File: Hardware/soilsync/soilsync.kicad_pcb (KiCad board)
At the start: 2 copper layers, 40 parts, among them J1 Barrel_Jack_Switch, J10 Screw_Terminal_01x03, J11 Screw_Terminal_01x03, J12 Screw_Terminal_01x03, J14 BMS_Terminal, J2 Screw_Terminal_01x03, J3 Screw_Terminal_01x03, J4 Screw_Terminal_01x03, J5 Screw_Terminal_01x03, J6 Screw_Terminal_01x03, J7 Screw_Terminal_01x03, J8 Screw_Terminal_01x03, J9 Screw_Terminal_01x03, U1 STM32F103C8Tx, U2 LM2596, U3 NRF24L01_Breakout, U4 AMS1117-3.3, U5 TP5100

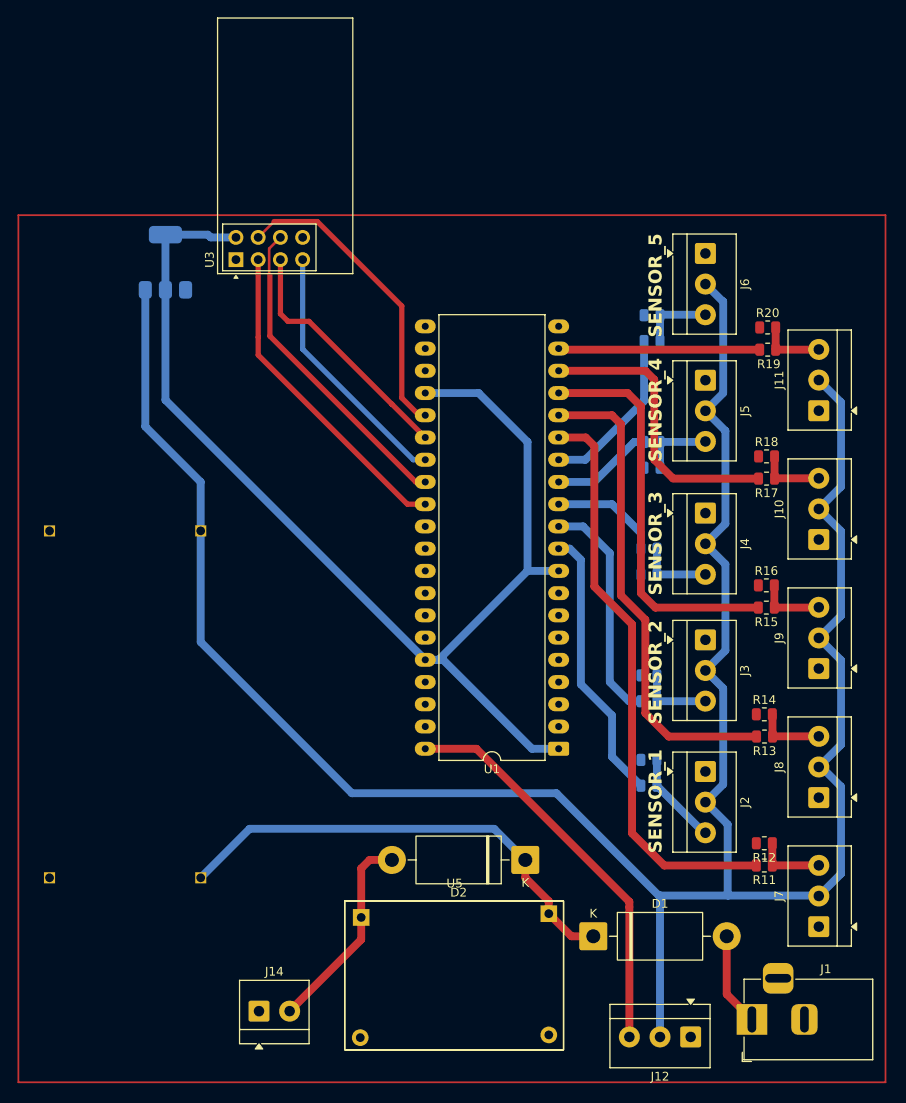
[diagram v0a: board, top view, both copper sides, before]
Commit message: PCB Finished
Generated fabrication data
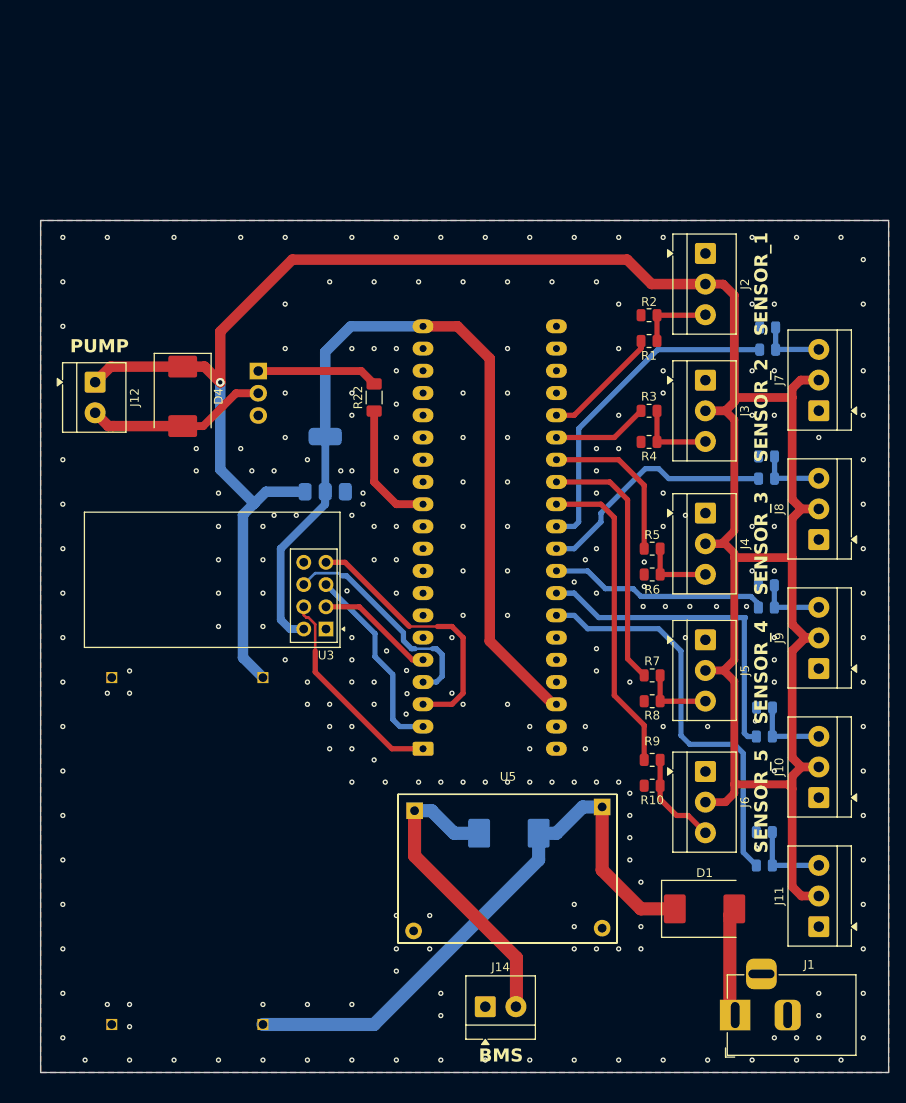
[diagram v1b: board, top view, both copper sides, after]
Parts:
- added D4: MBRS340, Diode_SMD:D_SMC, F.Cu at (183.9, 47.4)
- added Q1: IRLZ44N, Package_TO_SOT_THT:TO-220-3_Vertical, B.Cu at (192.5, 44.5)
- added R22: 100, Resistor_SMD:R_1206_3216Metric_Pad1.30x1.75mm_HandSolder, F.Cu at (205.7, 47.5)
- D1: value MBR340 -> MBRS340; footprint Diode_THT:D_DO-201AD_P15.24mm_Horizontal -> Diode_SMD:D_SMC
- D2: value MBR340 -> MBRS340; footprint Diode_THT:D_DO-201AD_P15.24mm_Horizontal -> Diode_SMD:D_SMC; moved to B.Cu
- J12: value Screw_Terminal_01x03 -> PUMP_Terminal; footprint TerminalBlock_4Ucon:TerminalBlock_4Ucon_1x03_P3.50mm_Horizontal -> TerminalBlock_4Ucon:TerminalBlock_4Ucon_1x02_P3.50mm_Horizontal
- R1, R10, R2, R3, R4, R5, R6, R7, R8, R9: moved to F.Cu
- R11, R12, R13, R14, R15, R16, R17, R18, R19, R20: moved to B.Cu
- U1: value STM32F103C8Tx -> YAAJ_BluePill; moved to B.Cu
- moved J12 101.1 mm to (173.9, 45.7), turned to -90 degrees
- moved J2 59.2 mm to (243.6, 31.0)
- moved J6 59.2 mm to (243.6, 90.2)
- moved J11 58.9 mm to (256.5, 108.0)
- moved J7 58.9 mm to (256.5, 49.0)
- moved R11 58.9 mm to (250.7, 42.0)
- moved R19 58.9 mm to (250.3, 101.0)
- moved R12 58.9 mm to (250.7, 39.5)
- moved R20 57.7 mm to (250.3, 97.2)
- moved R10 53.8 mm to (237.5, 91.8)
- moved R2 50.8 mm to (237.1, 38.1)
- moved R1 50.8 mm to (237.1, 41.0)
- moved R9 47.9 mm to (237.5, 88.9)
- moved U3 43.4 mm to (200.2, 74.0), turned to 180 degrees
- moved R3 33.2 mm to (237.1, 49.0)
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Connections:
- J12 pad 1: GND -> +5V
- J12 pad 2: +5V -> /PUMP-
- U1 pad 1: +3.3V -> /NRF_CSN
- U1 pad 10: SENSOR_1 -> unconnected-(U1-PA15-Pad10)
- U1 pad 11: SENSOR_2 -> unconnected-(U1-PB3-Pad11)
- U1 pad 12: SENSOR_3 -> /PUMP
- U1 pad 13: SENSOR_4 -> unconnected-(U1-PB5-Pad13)
- U1 pad 14: SENSOR_5 -> unconnected-(U1-PB6-Pad14)
- U1 pad 15: SENSOR_6 -> unconnected-(U1-PB7-Pad15)
- U1 pad 16: SENSOR_7 -> unconnected-(U1-PB8-Pad16)
- U1 pad 17: SENSOR_8 -> unconnected-(U1-PB9-Pad17)
- U1 pad 18: SENSOR_9 -> unconnected-(U1-5V-Pad18)
- U1 pad 19: SENSOR_10 -> GND
- U1 pad 2: unconnected-(U1-PC13-Pad2) -> /NRF_SCK
- U1 pad 20: unconnected-(U1-PB2-Pad20) -> +3.3V
- U1 pad 23: GND -> unconnected-(U1-PC14-Pad23)
- U1 pad 24: +3.3V -> unconnected-(U1-PC15-Pad24)
- U1 pad 25: /NRF_CSN -> SENSOR_1
- U1 pad 26: /NRF_SCK -> SENSOR_2
- U1 pad 27: /NRF_MISO -> SENSOR_3
- U1 pad 28: /NRF_MOSI -> SENSOR_4
- U1 pad 29: /NRF_CE -> SENSOR_5
- U1 pad 3: unconnected-(U1-PC14-Pad3) -> /NRF_MISO
- U1 pad 30: unconnected-(U1-PA9-Pad30) -> SENSOR_6
- U1 pad 31: unconnected-(U1-PA10-Pad31) -> SENSOR_7
- U1 pad 32: unconnected-(U1-PA11-Pad32) -> SENSOR_8
- U1 pad 33: unconnected-(U1-PA12-Pad33) -> SENSOR_9
- U1 pad 34: unconnected-(U1-PA13-Pad34) -> SENSOR_10
- U1 pad 35: GND -> unconnected-(U1-PB10-Pad35)
- U1 pad 36: +3.3V -> unconnected-(U1-PB11-Pad36)
- U1 pad 38: unconnected-(U1-PA15-Pad38) -> +3.3V
- U1 pad 39: unconnected-(U1-PB3-Pad39) -> GND
- U1 pad 4: unconnected-(U1-PC15-Pad4) -> /NRF_MOSI
- U1 pad 40: PUMP -> GND
- U1 pad 5: unconnected-(U1-PD0-Pad5) -> /NRF_CE
- U1 pad 8: GND -> unconnected-(U1-PA11-Pad8)
- U1 pad 9: +3.3V -> unconnected-(U1-PA12-Pad9)
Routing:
- net PUMP: track 46.0 -> 0.00 mm
- net +3.3V: track 136.7 -> 100.2 mm
- net SENSOR_6: track 66.2 -> 37.8 mm
- net SENSOR_7: track 55.5 -> 27.9 mm
- net SENSOR_10: track 23.2 -> 47.0 mm
- net /NRF_CE: track 37.0 -> 13.6 mm
- net /PUMP-: track 0.00 -> 20.8 mm
- net SENSOR_8: track 45.5 -> 25.1 mm
- net SENSOR_4: track 11.6 -> 29.8 mm
- net SENSOR_1: track 31.7 -> 13.7 mm
- net SENSOR_5: track 19.4 -> 36.3 mm
- net SENSOR_2: track 26.3 -> 10.9 mm
- net /PUMP: track 0.00 -> 14.7 mm
- net VIN: track 54.3 -> 68.2 mm
- net Net-(Q1-G): track 0.00 -> 13.9 mm
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- added copper zone on B.Cu, net GND
- added copper zone on F.Cu, net GND
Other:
- board outline added: 96.9 x 97.3 mm
- board text added: "BMS"
- board text added: "PUMP"
